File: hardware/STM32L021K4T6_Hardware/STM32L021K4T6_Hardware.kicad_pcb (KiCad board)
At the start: 2 copper layers, 60 x 50 mm, 27 parts, among them J1 Conn_02x07_Odd_Even, J2 INPUT, J3 POWER, J4 OUTPUT, U1 STM32L021K4Tx, U2 MCP1802x-xx02xOT, U3 MCP4801

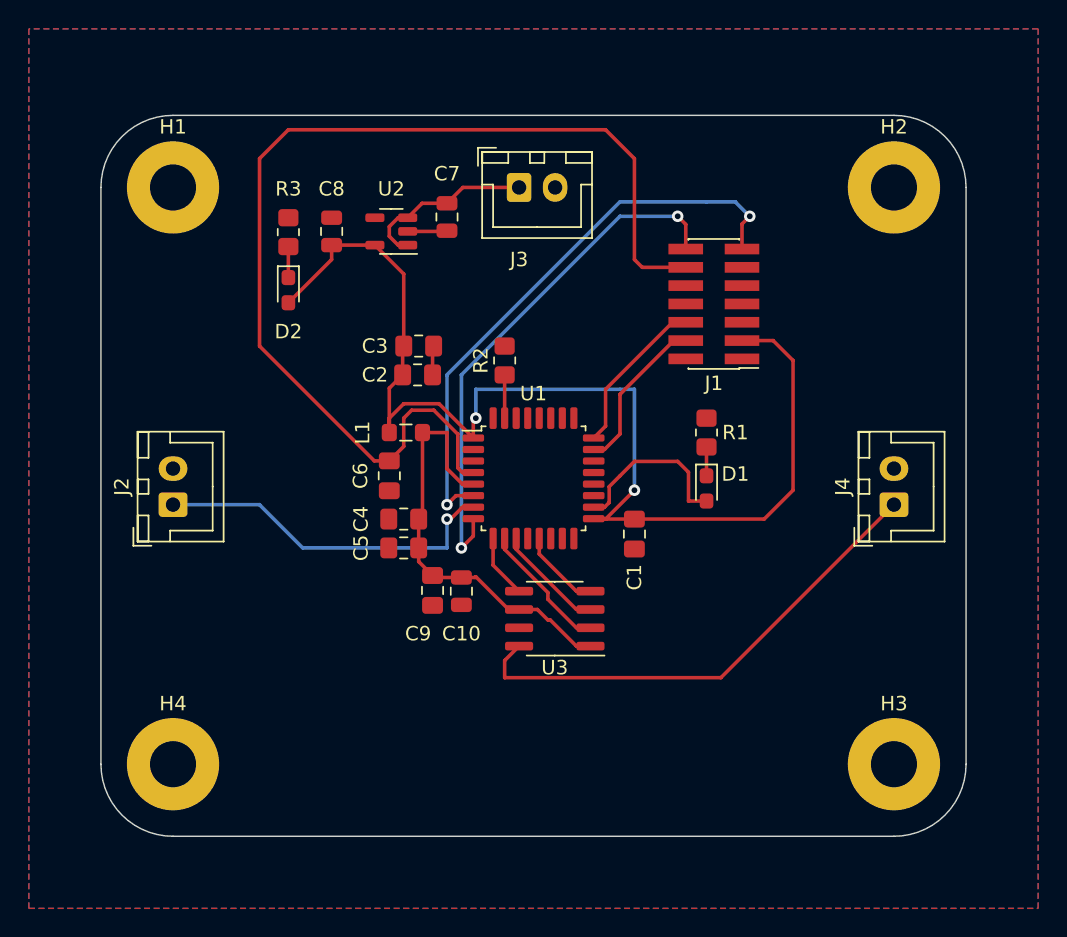
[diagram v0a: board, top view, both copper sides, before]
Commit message: drc check bis
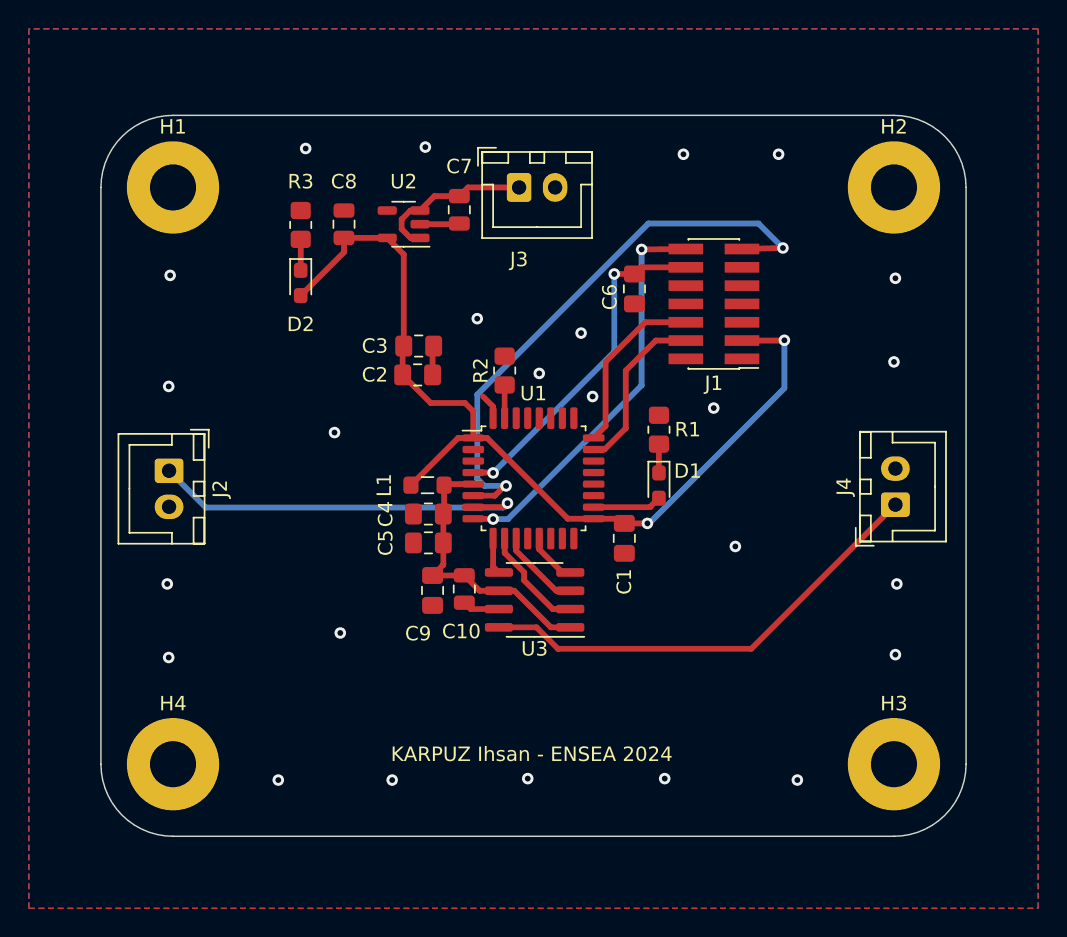
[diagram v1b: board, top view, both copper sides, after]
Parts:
- moved C6 21.4 mm to (162.0, 76.0)
- moved L1 3.95 mm to (147.7, 89.7)
- moved D1 3.31 mm to (163.7, 89.7)
- moved R1 3.31 mm to (163.7, 85.8)
- moved J2 2.37 mm to (129.7, 88.7), turned to -90 degrees
- moved U3 1.91 mm to (155.1, 97.6)
- moved C4 1.75 mm to (147.7, 91.7)
- moved C5 1.75 mm to (147.7, 93.7)
- moved U2 0.99 mm to (146.0, 71.5)
- moved C7 0.99 mm to (149.9, 70.5)
- moved C8 0.99 mm to (141.9, 71.5)
- moved D2 0.99 mm to (138.9, 75.6)
- moved R3 0.99 mm to (138.9, 71.6)
- moved C1 0.76 mm to (161.3, 93.3)
- moved R2 0.70 mm to (153.0, 81.7)
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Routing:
- net NRST: track 75.3 -> 23.9 mm, vias 0 -> 2
- net +3.3V: track 82.8 -> 66.0 mm
- net +3.3VA: track 30.1 -> 19.9 mm
- net USART2_TX: track 36.4 -> 28.1 mm
- net LED_STATUS: track 12.1 -> 4.78 mm
- net GND: track 4.78 -> 9.15 mm, vias 0 -> 25
- net ADC_IN1: track 24.5 -> 27.5 mm
- net DAC_OUT: track 34.6 -> 32.3 mm
- net SPI1_MOSI: track 5.69 -> 3.56 mm
- net DAC_nLDAC: track 4.40 -> 2.52 mm
- net SPI1_SCK: track 7.62 -> 5.75 mm
- net DAC_nCS: track 9.23 -> 7.48 mm
- net SWDCK: track 11.2 -> 12.3 mm
- net +5V: track 12.3 -> 11.3 mm
- net SWDIO: track 11.1 -> 11.9 mm
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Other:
- board text added: "KARPUZ Ihsan - ENSEA 2024"
